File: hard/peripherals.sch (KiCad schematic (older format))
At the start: 9 parts, among them J3 PJ-3062-CO, U2 ADXL345BCCZ-RL7

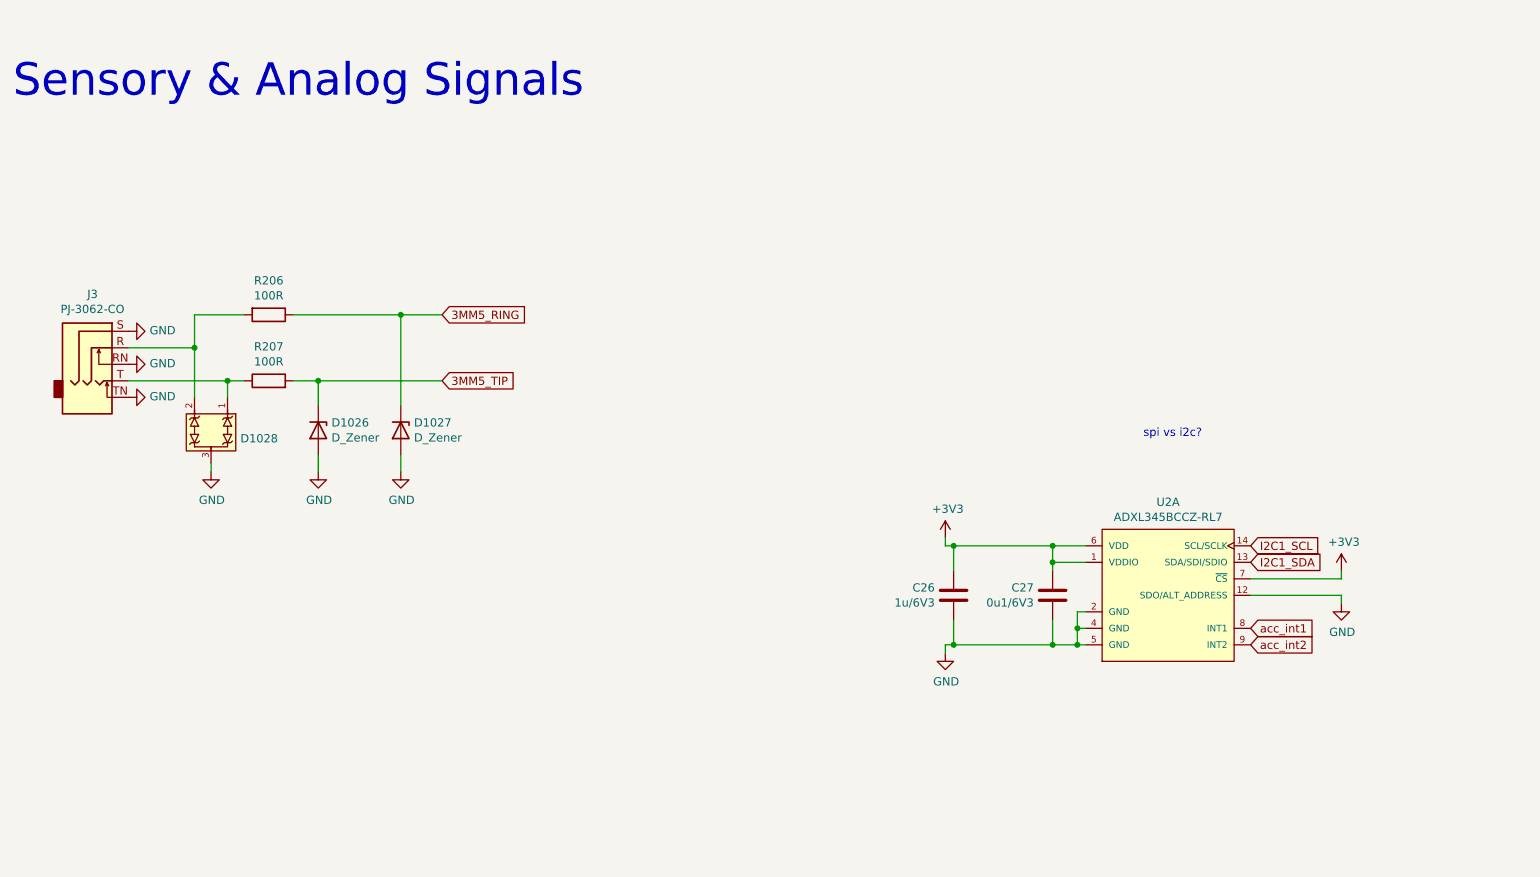
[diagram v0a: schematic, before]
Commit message: layout process
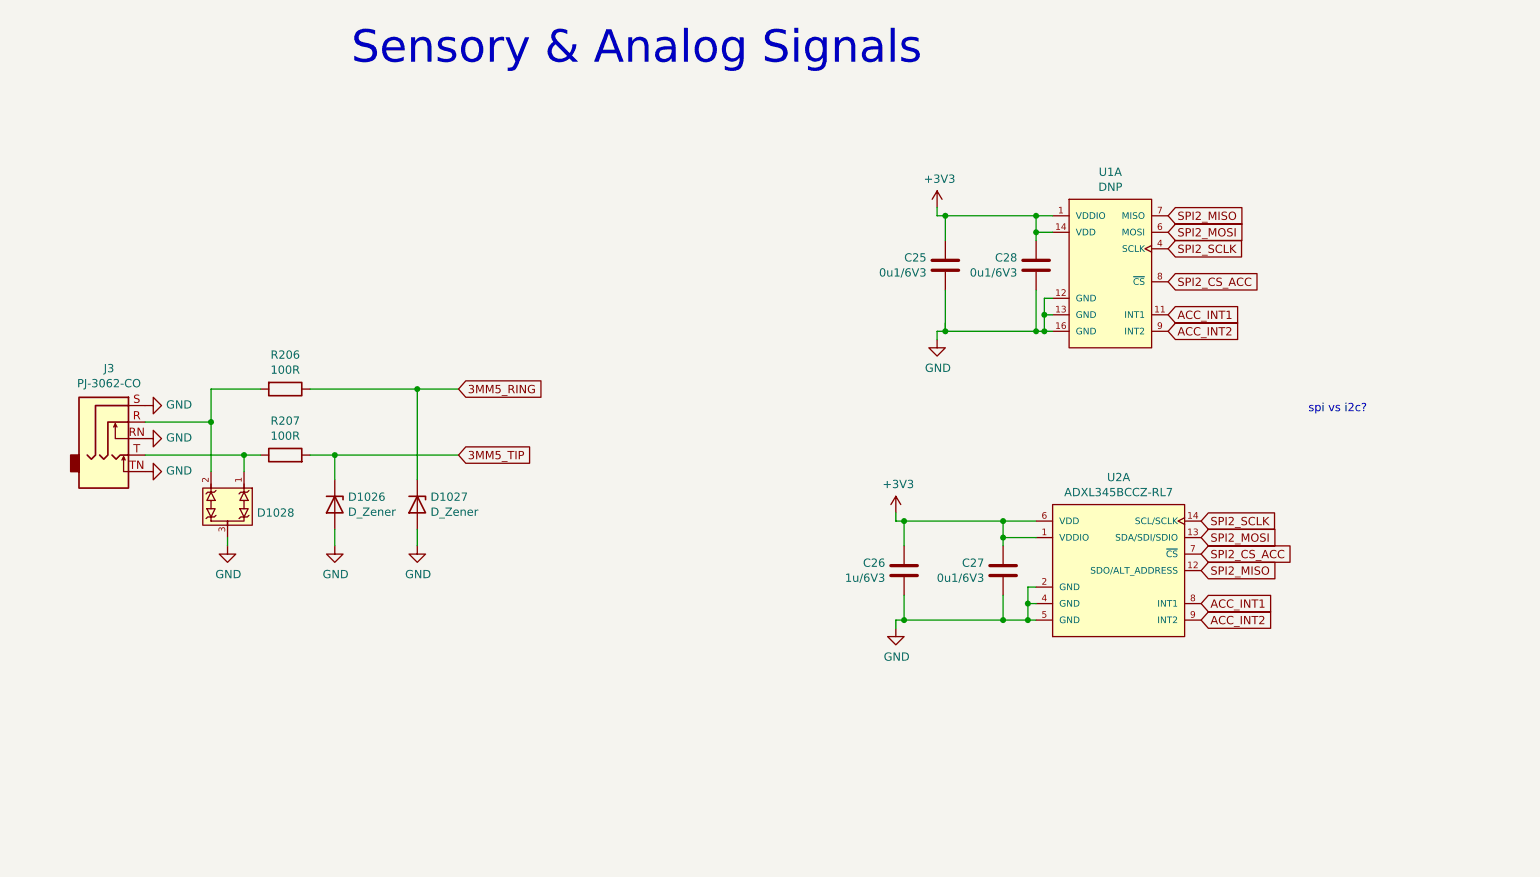
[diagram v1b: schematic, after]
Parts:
- added C25, C28: 0u1/6V3, Capacitor_SMD:C_0402_1005Metric, symbol Device:C
- added U1: DNP, led_matrix:Sensors_AnalogDevices_ADXL362BCCZ-RX, symbol led_matrix:ADXL362BCCZ-RLX
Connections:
- net +3V3: now also C25.2, C28.2, U1.1 (VDDIO), U1.14 (VDD); no longer U2.7 (~CS~)
- net GND: now also C25.1, C28.1, U1.12 (GND), U1.13 (GND), U1.16 (GND); no longer U2.12 (SDO/ALT_ADDRESS)
- net I2C1_SCL renamed SPI2_SCLK
- net SPI2_SCLK: now also U1.4 (SCLK)
- net I2C1_SDA renamed SPI2_MOSI
- net SPI2_MOSI: now also U1.6 (MOSI)
- net acc_int1 renamed ACC_INT1
- net ACC_INT1: now also U1.11 (INT1)
- net acc_int2 renamed ACC_INT2
- net ACC_INT2: now also U1.9 (INT2)
- new net SPI2_CS_ACC: U1.8 (~CS~), U2.7 (~CS~)
- new net SPI2_MISO: U1.7 (MISO), U2.12 (SDO/ALT_ADDRESS)
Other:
- moved on the sheet: C26, C27, D1026, D1027, D1028, J3, R206, R207, U2A

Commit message: release candidate. ready for review by @lukekaese
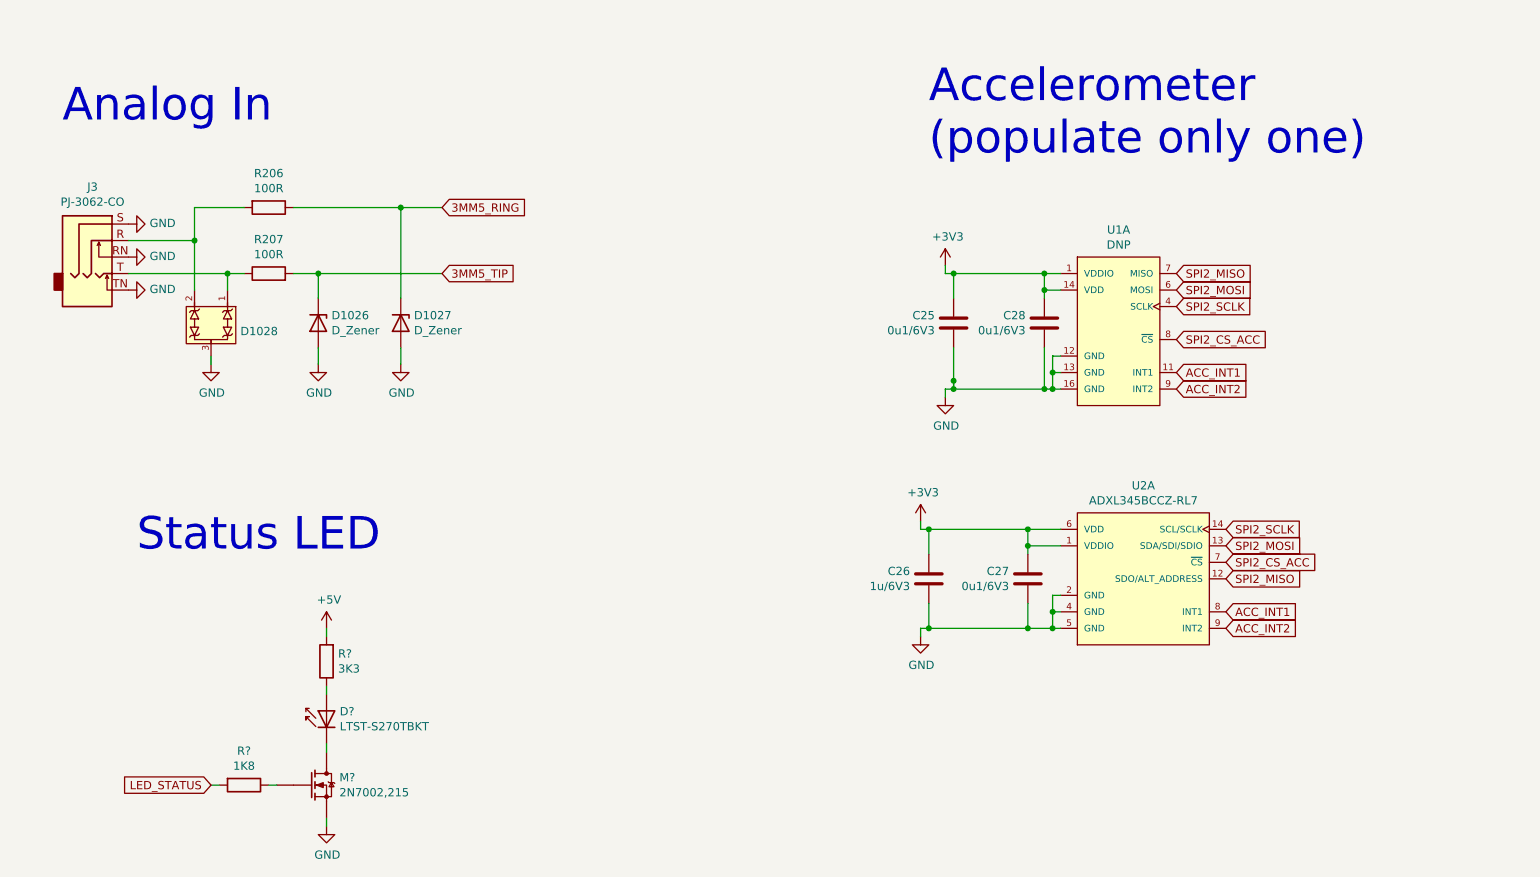
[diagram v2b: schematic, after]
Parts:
- added D?: LTST-S270TBKT, led_matrix:LED_LiteOn_LTST-S270TBKT, symbol led_matrix:LTST-S270TBKT
- added M?: 2N7002,215, Package_TO_SOT_SMD:SOT-23, symbol led_matrix:2N7002,215
- added R?: 3K3, Resistor_SMD:R_0402_1005Metric, symbol Device:R
- added R?: 1K8, Resistor_SMD:R_0402_1005Metric, symbol Device:R
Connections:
- net GND: now also M?.2 (S)
- new net: D?.A, R?.1
- new net: D?.C, M?.3 (D)
- new net: M?.1 (G), R?.1
- new net +5V: R?.2
- new net LED_STATUS: R?.2
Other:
- note added: "Accelerometer\n(populate only one)"
- note added: "Analog In"
- note added: "Status LED"
- note removed: "Sensory & Analog Signals"
- note removed: "spi vs i2c?"
- moved on the sheet: C25, C26, C27, C28, D1026, D1027, D1028, J3, R206, R207, U1A, U2A
